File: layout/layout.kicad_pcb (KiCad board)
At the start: 2 copper layers, 2 parts

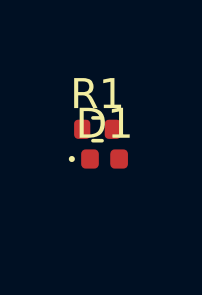
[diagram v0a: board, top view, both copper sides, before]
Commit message: layout testing
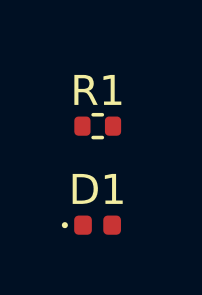
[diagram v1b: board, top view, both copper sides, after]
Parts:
- moved D1 2.22 mm to (148.4, 107.7)
- moved R1 0.11 mm to (148.4, 104.4)
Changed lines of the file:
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@@
 	(footprint "LED_0402_1005Metric:LED_0402_1005Metric"
 		(layer "F.Cu")
-		(at 148.6175 105.495)
+		(at 148.385 107.7)
 		(descr "LED SMD 0402 (1005 Metric), square (rectangular) end terminal, IPC_7351 nominal, (Body size source: http://www.tortai-tech.com/upload/download/2011102023233369053.pdf), generated with kicad-footprint-generator")
 		(tags "LED")
@@
 			)
 		)
+		(property "Type" "led"
+			(at 0 0 0)
+			(layer "F.SilkS")
+			(hide yes)
+			(effects
+				(font
+					(size 1.27 1.27)
+					(thickness 0.15)
+				)
+			)
+		)
+		(property "symbol_path" "/Users/garyfodi/Library/Caches/pcb/gitlab/kicad/libraries/kicad-symbols/9.0.0/Device.kicad_sym"
+			(at 0 0 0)
+			(layer "F.SilkS")
+			(hide yes)
+			(effects
+				(font
+					(size 1.27 1.27)
+					(thickness 0.15)
+				)
+			)
+		)
+		(property "symbol_name" "LED_Small_Filled"
+			(at 0 0 0)
+			(layer "F.SilkS")
+			(hide yes)
+			(effects
+				(font
+					(size 1.27 1.27)
+					(thickness 0.15)
+				)
+			)
+		)
 		(property "prefix" "D"
 			(at 0 0 0)
@@
 		)
 		(property "Color" "red"
-			(at 0 0 0)
-			(layer "F.SilkS")
-			(hide yes)
-			(effects
-				(font
-					(size 1.27 1.27)
-					(thickness 0.15)
-				)
-			)
-		)
-		(property "symbol_name" "LED_Small_Filled"
-			(at 0 0 0)
-			(layer "F.SilkS")
-			(hide yes)
-			(effects
-				(font
-					(size 1.27 1.27)
-					(thickness 0.15)
-				)
-			)
-		)
-		(property "symbol_path" "/Users/garyfodi/Library/Caches/pcb/gitlab/kicad/libraries/kicad-symbols/9.0.0/Device.kicad_sym"
-			(at 0 0 0)
-			(layer "F.SilkS")
-			(hide yes)
-			(effects
-				(font
-					(size 1.27 1.27)
-					(thickness 0.15)
-				)
-			)
-		)
-		(property "Type" "led"
 			(at 0 0 0)
 			(layer "F.SilkS")
@@
 	(footprint "R_0402_1005Metric:R_0402_1005Metric"
 		(layer "F.Cu")
-		(at 148.3825 104.505)
+		(at 148.39 104.4)
 		(descr "Resistor SMD 0402 (1005 Metric), square (rectangular) end terminal, IPC_7351 nominal, (Body size source: IPC-SM-782 page 72, https://www.pcb-3d.com/wordpress/wp-content/uploads/ipc-sm-782a_amendment_1_and_2.pdf), generated with kicad-footprint-generator")
 		(tags "resistor")
@@
 			)
 		)
+		(property "Type" "resistor"
+			(at 0 0 0)
+			(layer "F.SilkS")
+			(hide yes)
+			(effects
+				(font
+					(size 1.27 1.27)
+					(thickness 0.15)
+				)
+			)
+		)
+		(property "Package" "0402"
+			(at 0 0 0)
+			(layer "F.SilkS")
+			(hide yes)
+			(effects
+				(font
+					(size 1.27 1.27)
+					(thickness 0.15)
+				)
+			)
+		)
+		(property "prefix" "R"
+			(at 0 0 0)
+			(layer "F.SilkS")
+			(hide yes)
+			(effects
+				(font
+					(size 1.27 1.27)
+					(thickness 0.15)
+				)
+			)
+		)
 		(property "symbol_name" "R"
 			(at 0 0 0)
@@
 			)
 		)
-		(property "Type" "resistor"
-			(at 0 0 0)
-			(layer "F.SilkS")
-			(hide yes)
-			(effects
-				(font
-					(size 1.27 1.27)
-					(thickness 0.15)
-				)
-			)
-		)
-		(property "Package" "0402"
+		(property "symbol_path" "/Users/garyfodi/Library/Caches/pcb/gitlab/kicad/libraries/kicad-symbols/9.0.0/Device.kicad_sym"
 			(at 0 0 0)
 			(layer "F.SilkS")
@@
 			(at 0 0 0)
 			(layer "F.SilkS")
-			(hide yes)
-			(effects
-				(font
-					(size 1.27 1.27)
-					(thickness 0.15)
-				)
-			)
-		)
-		(property "symbol_path" "/Users/garyfodi/Library/Caches/pcb/gitlab/kicad/libraries/kicad-symbols/9.0.0/Device.kicad_sym"
-			(at 0 0 0)
-			(layer "F.SilkS")
-			(hide yes)
-			(effects
-				(font
-					(size 1.27 1.27)
-					(thickness 0.15)
-				)
-			)
-		)
-		(property "prefix" "R"
-			(at 0 0 0)
-			(layer "F.SilkS")

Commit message: patch for widget
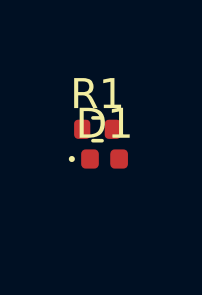
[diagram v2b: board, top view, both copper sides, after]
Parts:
- moved D1 2.22 mm to (148.6, 105.5)
- moved R1 0.11 mm to (148.4, 104.5)
